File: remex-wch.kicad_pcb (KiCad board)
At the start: 4 copper layers, 83.8 x 22.9 mm, 99 parts, among them J1 Conn_01x16, J2 Conn_01x12, J3 USB_C_Receptacle_USB2.0_16P, J4 Micro_SD_Card_Det1, J5 RJ45_Hanrun_HR911130C, J7 JST_PH, SW1 RESET, U1 CH32V307WCU6, U2 RTL8211F, U3 MS5351M, U4 HUSB311, U5 SY6820, U6 LW52xxN11E, U7 LGS5500, U8 PY32F002AW15U, Y1 32.768kHz 12.5 pF Q13FC135000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, Y2 25 MHz 10 pF X322525MMB4SI

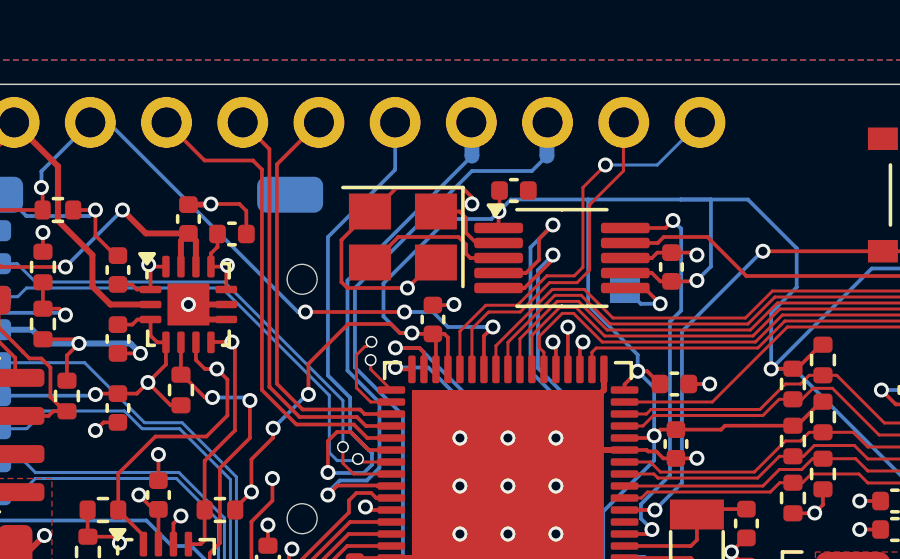
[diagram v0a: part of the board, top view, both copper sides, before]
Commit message: hopefully fix nettie
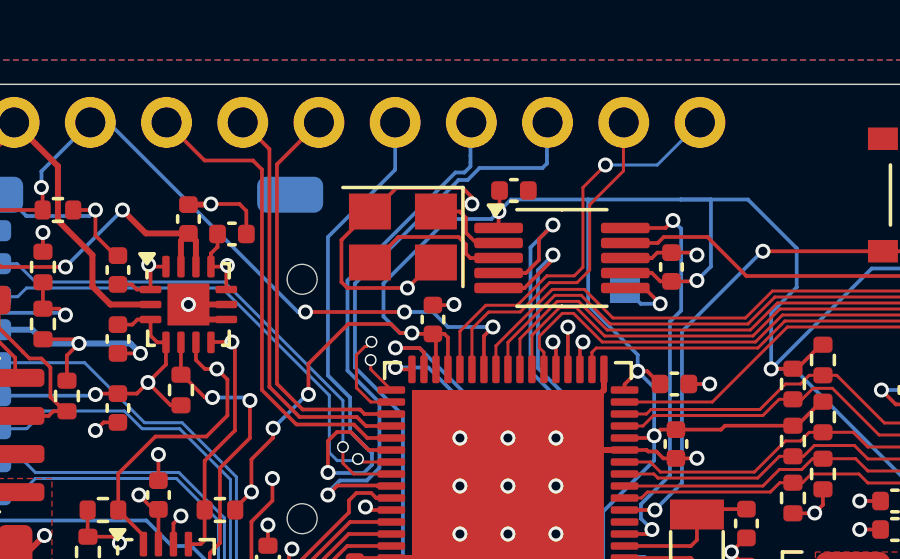
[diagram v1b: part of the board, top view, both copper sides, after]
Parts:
- NT1, NT2: footprint NetTie:NetTie-2_SMD_Pad0.5mm -> parts:nettie_tiny
- moved NT1 0.60 mm to (81.2, 133.3)
- moved NT2 0.60 mm to (83.8, 133.3)
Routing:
- net /EXT_D6: track 0.00 -> 1.11 mm
- net /EXT_D5: track 0.00 -> 1.10 mm
